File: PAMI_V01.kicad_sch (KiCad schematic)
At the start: 49 parts, among them J10 Conn_01x07, J2 Conn, J20 Conn_01x03, J21 Conn_01x03, J22 Conn_01x02, J3 Conn_OLED_Screen, J4 Conn_01x04, J4 USB_B, J5 Conn_02x02_Odd_Even, J6 Conn_02x02_Odd_Even, J7 Conn_01x04, J7 PAMI_Type, J8 Conn_01x02, J9 Conn_01x07, M1 Motor_Servo, M2 Motor_Servo, SW3 EN, SW4 BAU, SW4 TRT, U1 ESP32-S3-WROOM-1, U2 TMC2209_SILENTSTEPSTICK, U4 TMC2209_SILENTSTEPSTICK, U5 TSR_2-2433

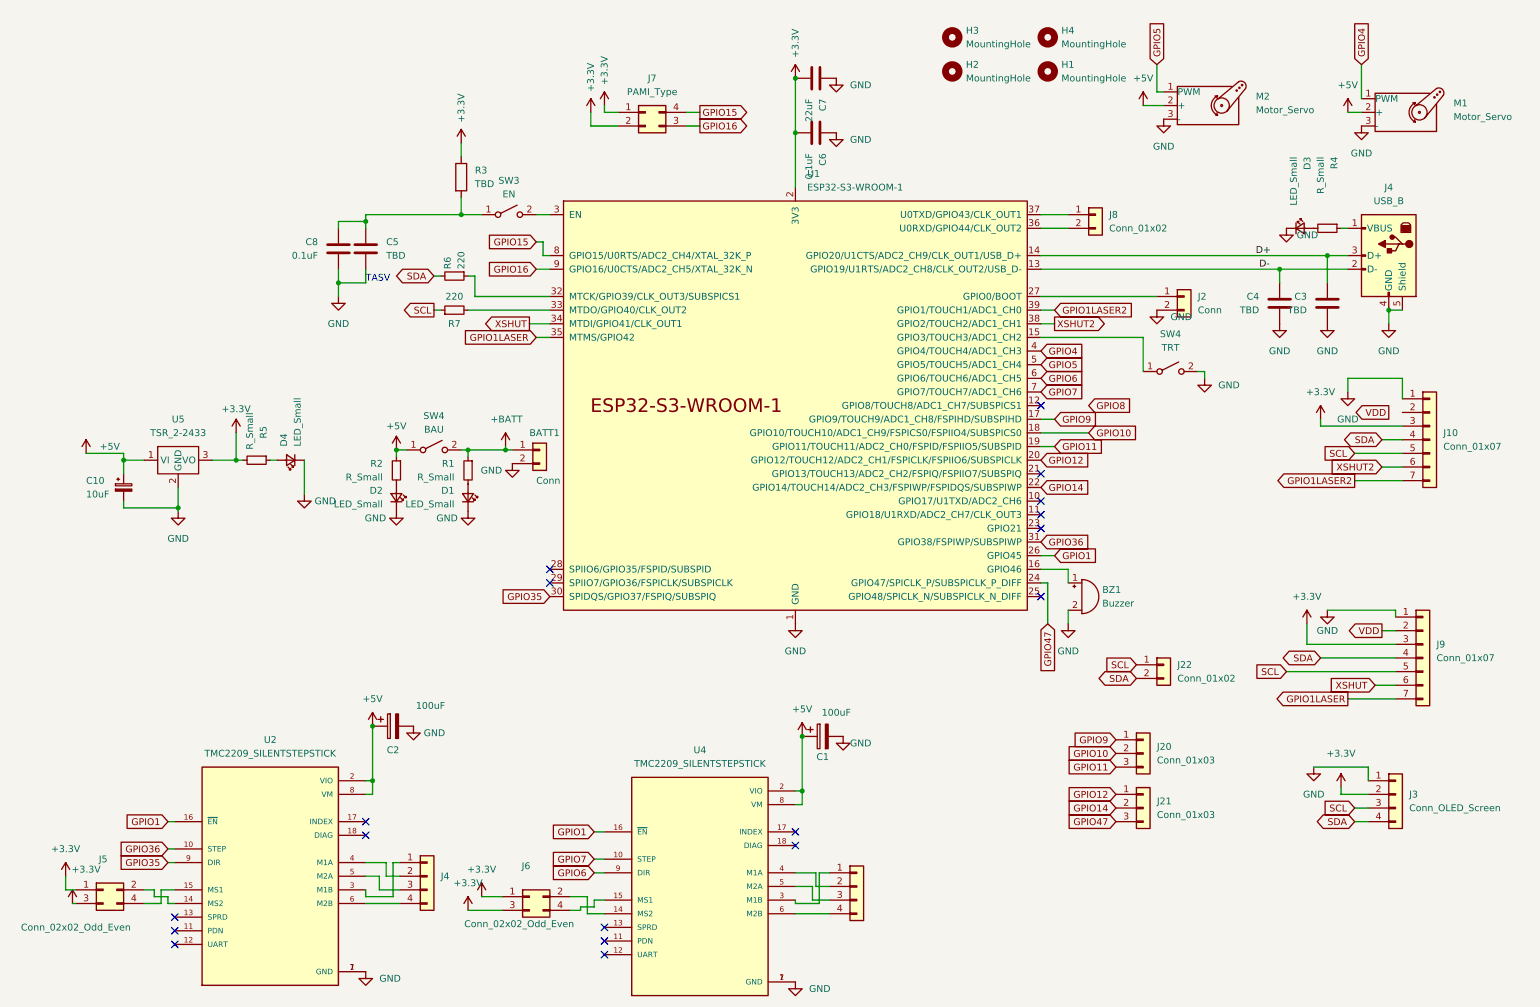
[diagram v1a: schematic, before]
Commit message: Unishape PAMI board V2
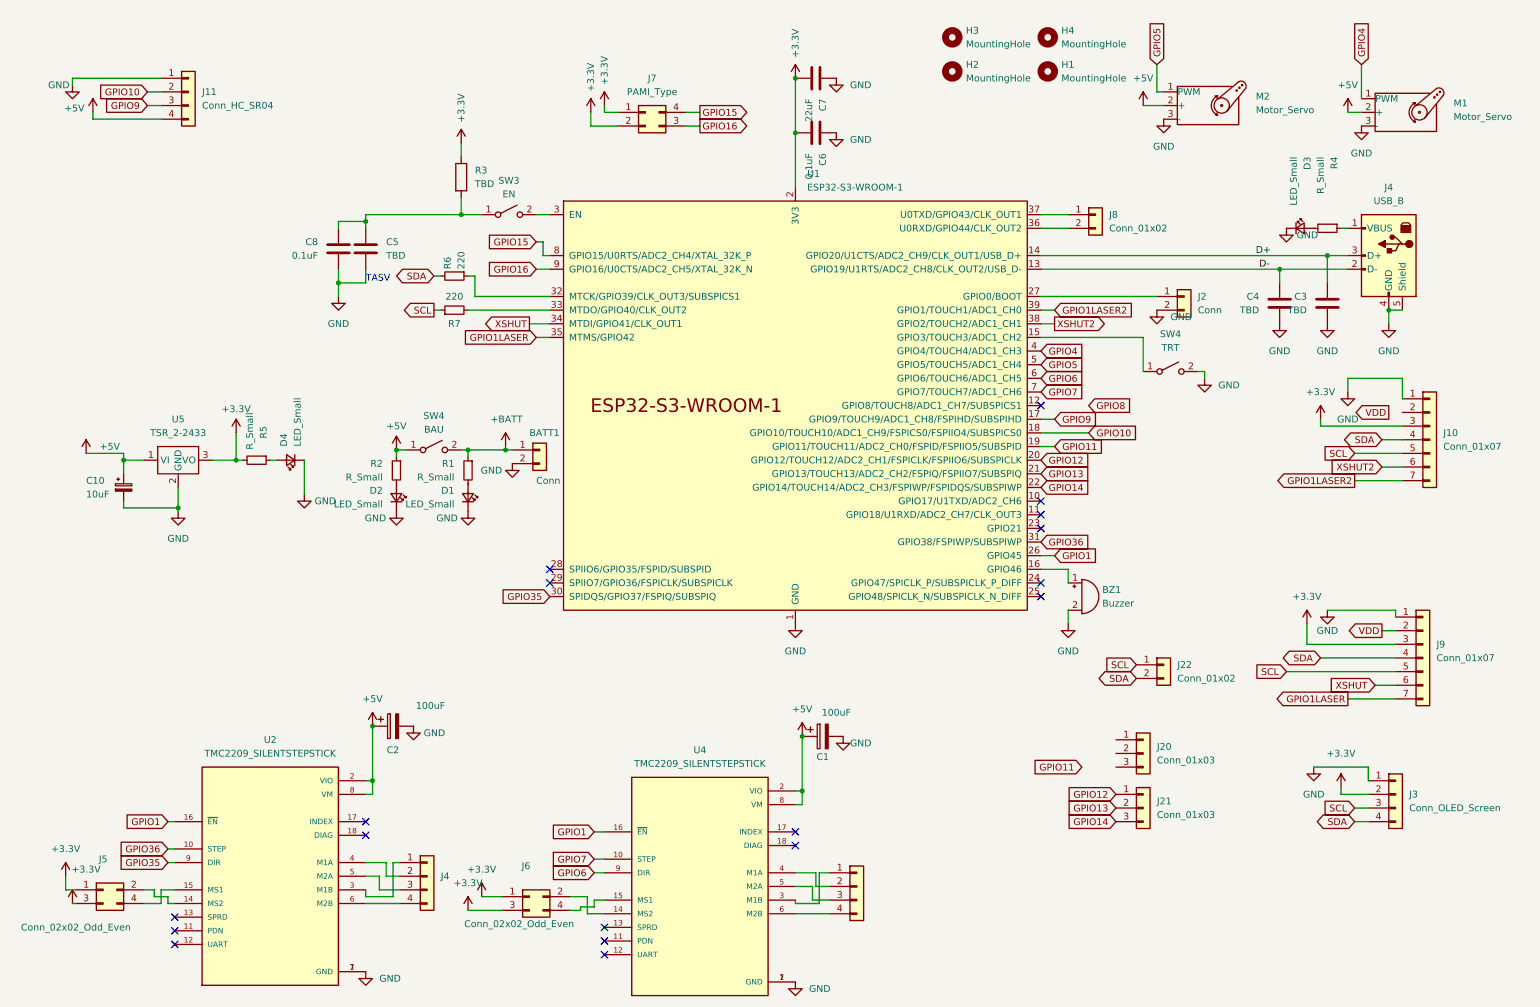
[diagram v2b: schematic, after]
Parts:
- added J11: Conn_HC_SR04, Connector_PinHeader_2.54mm:PinHeader_1x04_P2.54mm_Vertical, symbol Connector_Generic:Conn_01x04
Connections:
- net +5V: now also J11.4 (Pin_4)
- net GND: now also J11.1 (Pin_1)
- net GPIO10: now also J11.2 (Pin_2); no longer J20.2 (Pin_2)
- net GPIO11: no longer J20.3 (Pin_3)
- net GPIO14: now also J21.3 (Pin_3); no longer J21.2 (Pin_2)
- net GPIO9: now also J11.3 (Pin_3); no longer J20.1 (Pin_1)
- net GPIO13: now reaches U1.21 (GPIO13/TOUCH13/ADC2_CH2/FSPIQ/FSPIIO7/SUBSPIQ)
- net GPIO13: now also J21.2 (Pin_2)
- net GPIO47: no longer names the net of U1.24 (GPIO47/SPICLK_P/SUBSPICLK_P_DIFF)
- net GPIO47: no longer J21.3 (Pin_3)
